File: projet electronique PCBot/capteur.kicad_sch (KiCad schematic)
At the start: 3 parts, among them J2 nRF24, J3 TOF, U5 LSM6DSOX

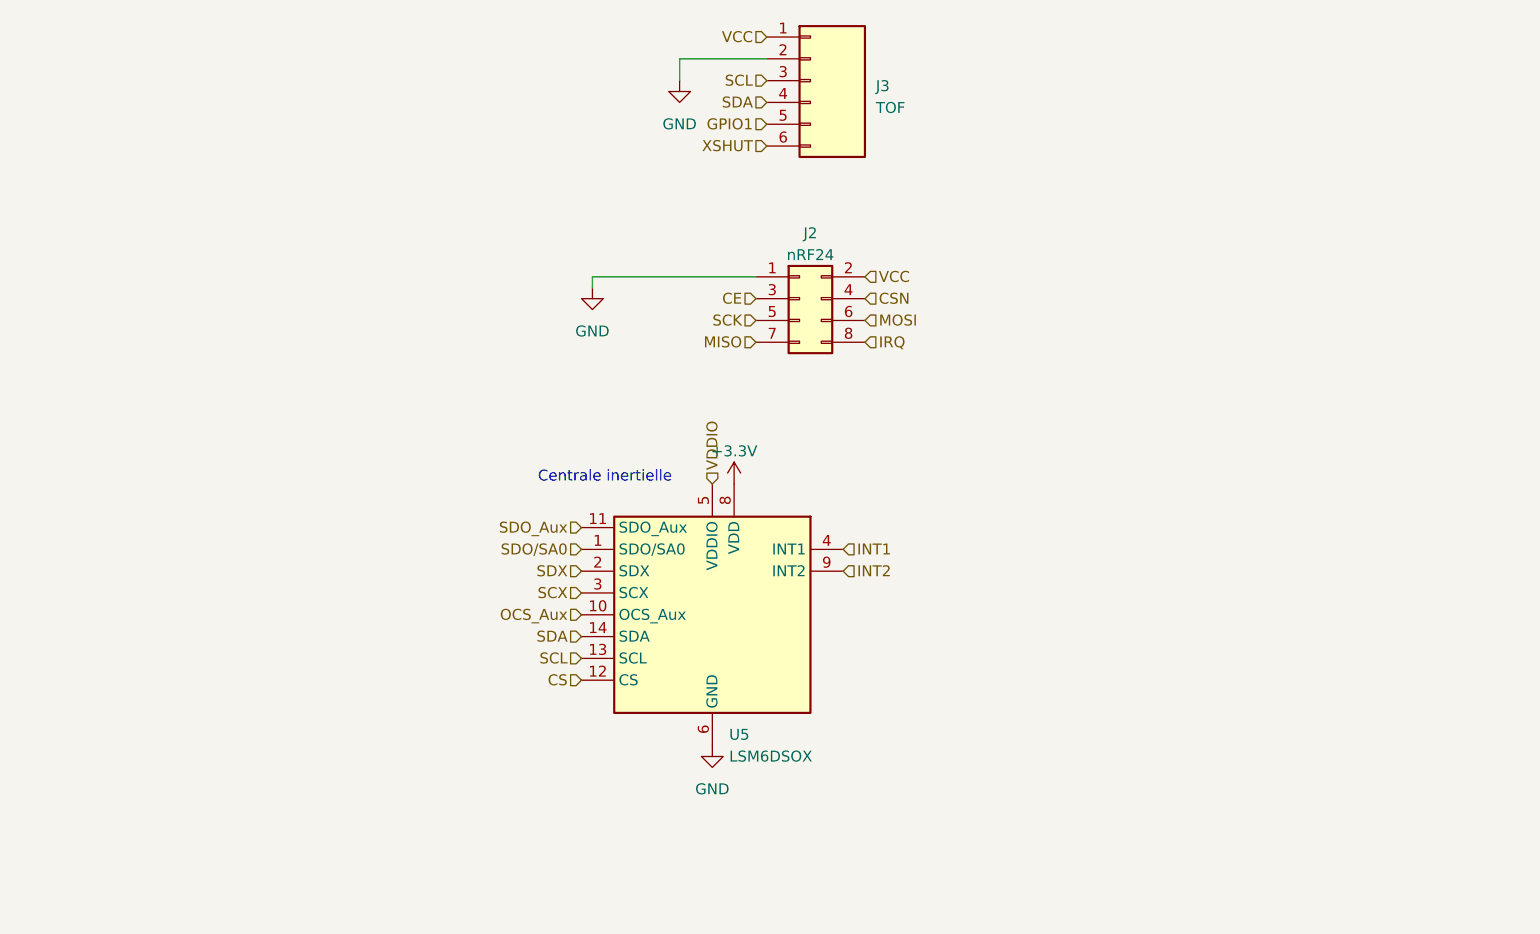
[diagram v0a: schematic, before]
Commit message: modification de la feuille capteurs
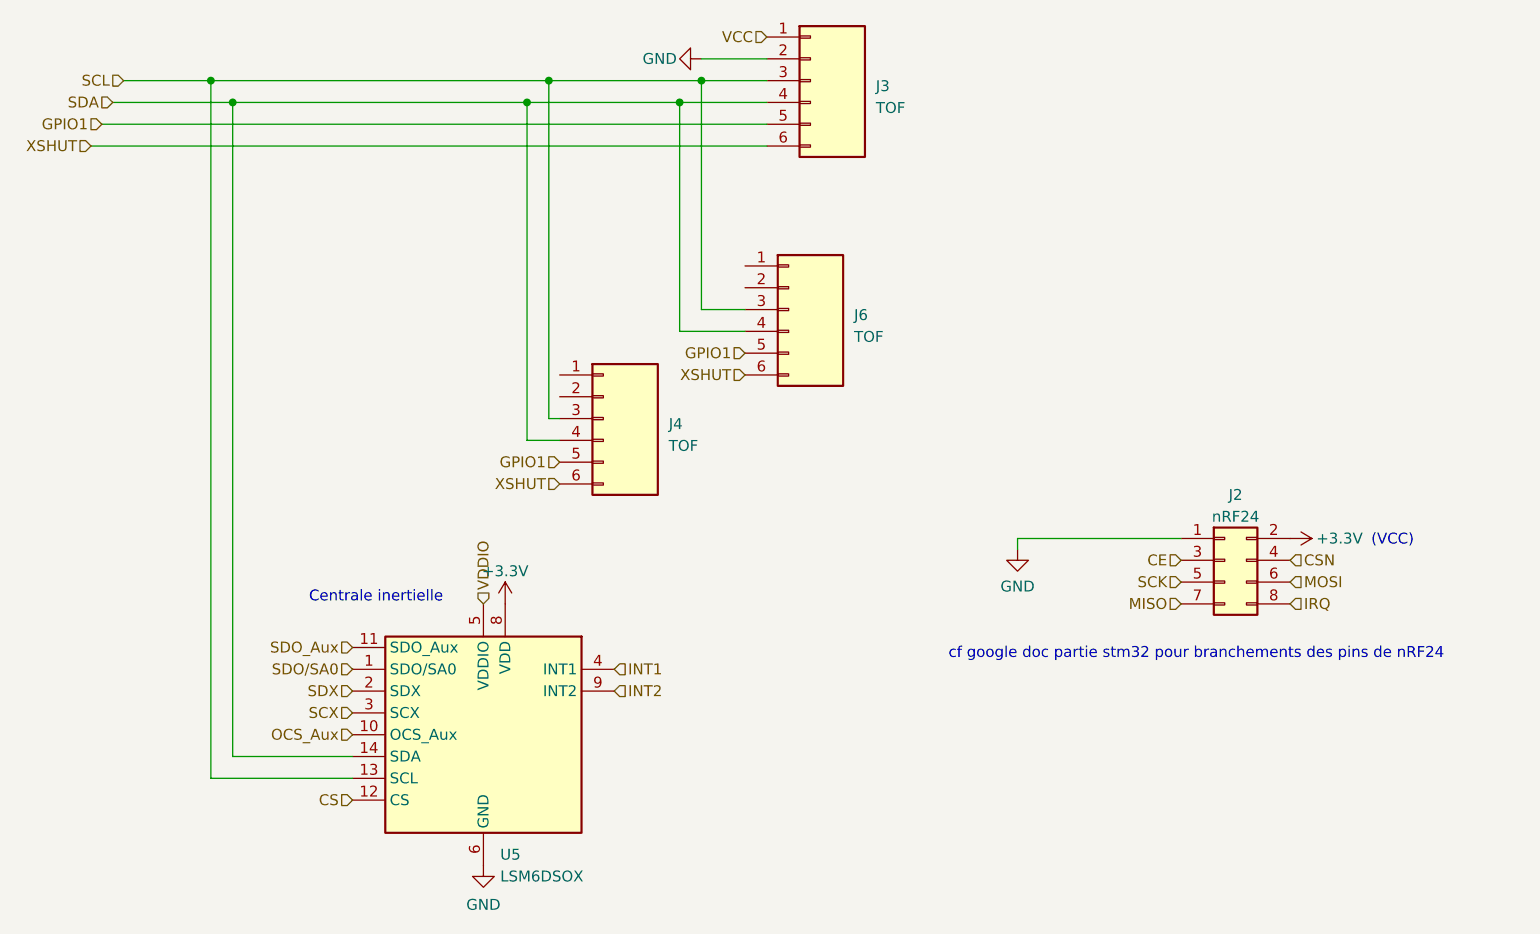
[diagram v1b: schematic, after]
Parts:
- added J4, J6: TOF, symbol pcbot_lib:TOF
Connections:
- net +3.3V: now also J2.2 (Pin_2)
- net GPIO1: now also J4.5 (GPIO1), J6.5 (GPIO1)
- net SCL: now also J4.3 (SCL), J6.3 (SCL)
- net SDA: now also J4.4 (SDA), J6.4 (SDA)
- net VCC: no longer J2.2 (Pin_2)
- net XSHUT: now also J4.6 (XST), J6.6 (XST)
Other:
- note added: "(VCC)"
- note added: "cf google doc partie stm32 pour branchements des pins de nRF24"
- moved on the sheet: J2, U5
